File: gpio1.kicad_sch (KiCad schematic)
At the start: 2 parts, among them U27 RK3576

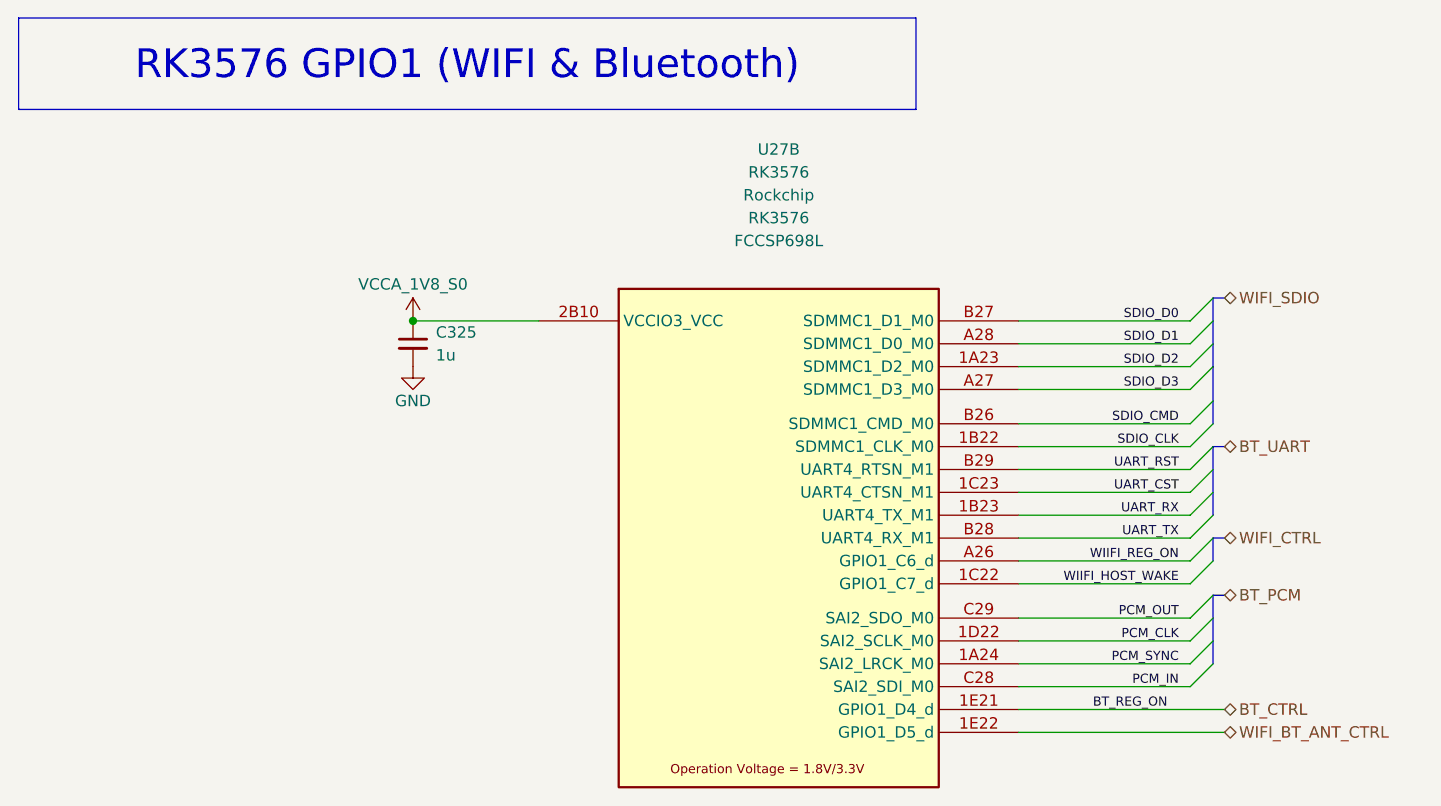
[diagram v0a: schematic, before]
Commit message: Add files via upload
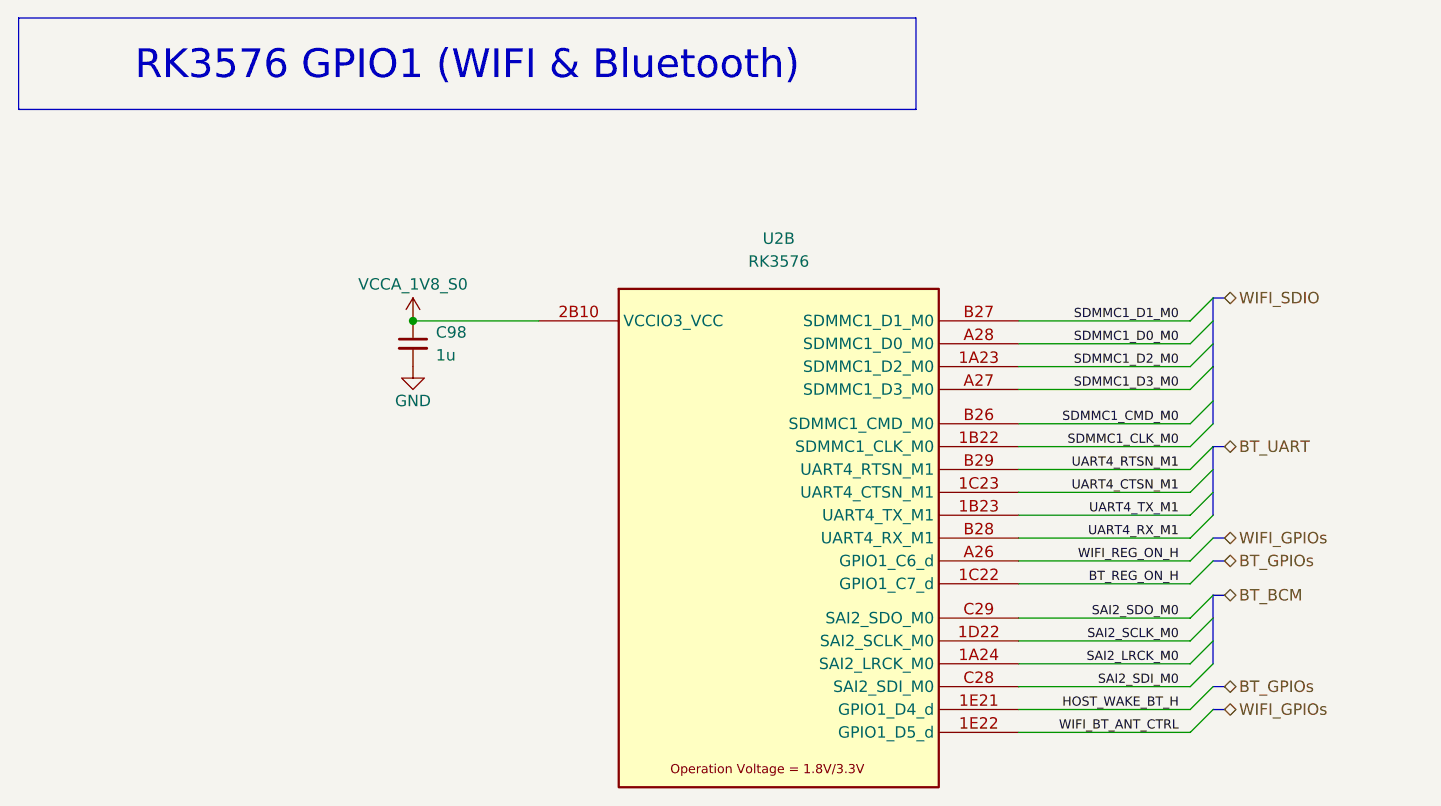
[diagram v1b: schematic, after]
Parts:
- renumbered C325 to C98, U27 to U2
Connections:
- net BT_CTRL renamed HOST_WAKE_BT_H
- net PCM_CLK renamed SAI2_SCLK_M0
- net PCM_IN renamed SAI2_SDI_M0
- net PCM_OUT renamed SAI2_SDO_M0
- net PCM_SYNC renamed SAI2_LRCK_M0
- net SDIO_CLK renamed SDMMC1_CLK_M0
- net SDIO_CMD renamed SDMMC1_CMD_M0
- net SDIO_D0 renamed SDMMC1_D1_M0
- net SDIO_D1 renamed SDMMC1_D0_M0
- net SDIO_D2 renamed SDMMC1_D2_M0
- net SDIO_D3 renamed SDMMC1_D3_M0
- net UART_CST renamed UART4_CTSN_M1
- net UART_RST renamed UART4_RTSN_M1
- net UART_RX renamed UART4_TX_M1
- net UART_TX renamed UART4_RX_M1
- net WIIFI_HOST_WAKE renamed BT_REG_ON_H
- net WIIFI_REG_ON renamed WIFI_REG_ON_H
